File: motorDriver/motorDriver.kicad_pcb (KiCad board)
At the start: 2 copper layers, 20.1 x 21.3 mm, 8 parts, among them P1 Vcc, P2 Input, P3 Output, U1 TB6593FNG

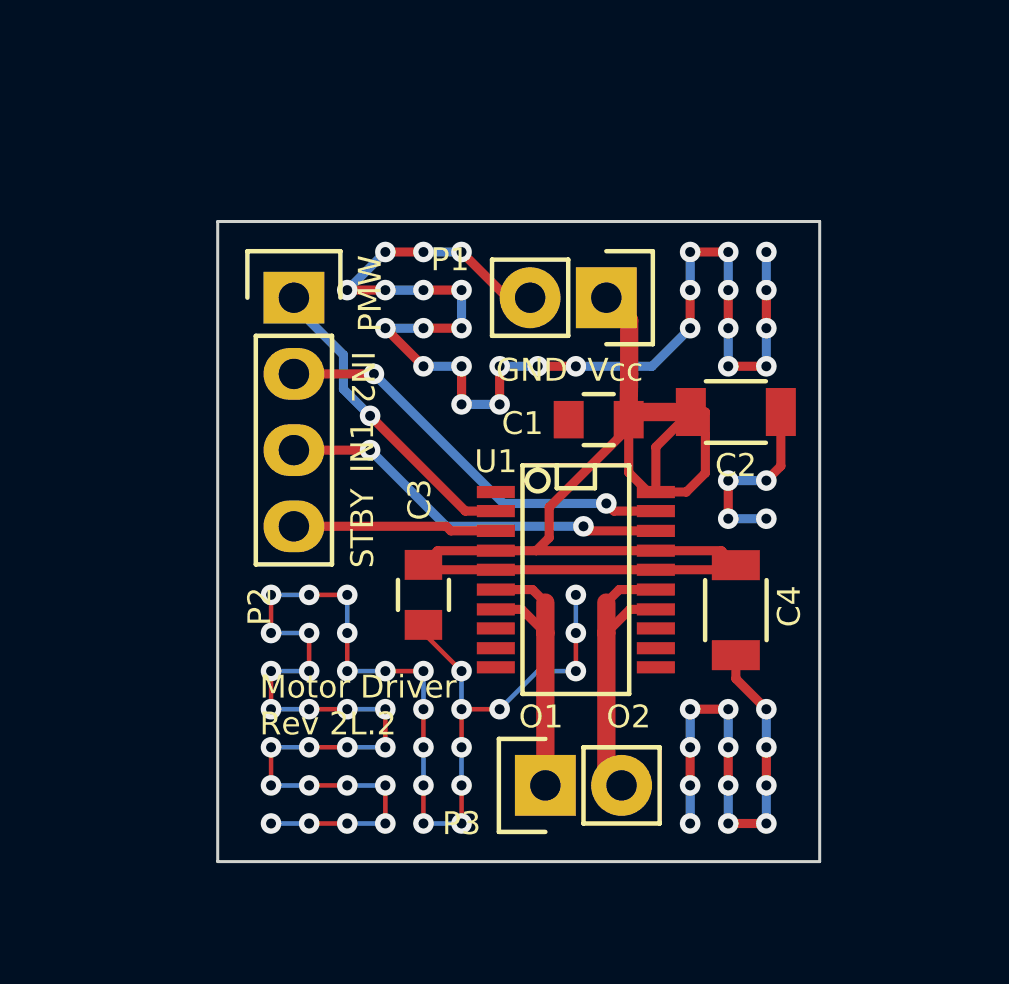
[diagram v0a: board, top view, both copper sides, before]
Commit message: Updated layout for Rev 2
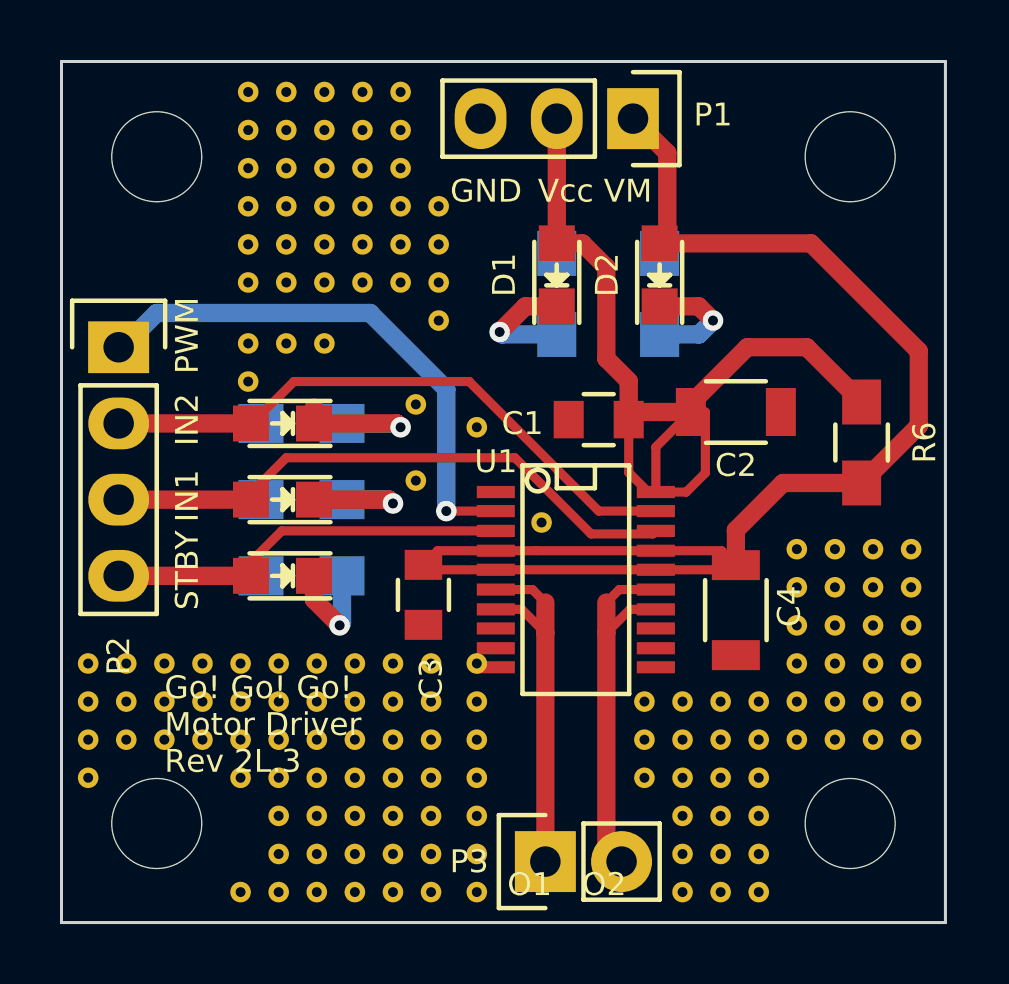
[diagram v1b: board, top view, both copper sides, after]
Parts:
- added D1: LED, LEDs:LED-0805, F.Cu at (159.4, 82.0)
- added D2: LED, LEDs:LED-0805, F.Cu at (162.8, 82.0)
- added D3: LED, LEDs:LED-0805, F.Cu at (150.2, 92.1)
- added IN1: LED, LEDs:LED-0805, F.Cu at (150.2, 89.5)
- added IN2: LED, LEDs:LED-0805, F.Cu at (150.2, 87.0)
- added R1: 1KΩ, Resistors_SMD:R_0805_HandSoldering, B.Cu at (159.4, 82.7)
- added R2: 1KΩ, Resistors_SMD:R_0805_HandSoldering, B.Cu at (162.8, 82.7)
- added R3: 1KΩ, Resistors_SMD:R_0805_HandSoldering, B.Cu at (150.9, 89.5)
- added R4: 1KΩ, Resistors_SMD:R_0805_HandSoldering, B.Cu at (150.9, 87.0)
- added R5: 1KΩ, Resistors_SMD:R_0805_HandSoldering, B.Cu at (150.9, 92.1)
- added R6: 0Ω, Resistors_SMD:R_0805_HandSoldering, F.Cu at (169.5, 87.6)
- added REF**: MountingHole_3mm, Mounting_Holes:MountingHole_3mm, F.Cu at (169.2, 100.3)
- added REF**: MountingHole_3mm, Mounting_Holes:MountingHole_3mm, F.Cu at (146.1, 100.3)
- added REF**: MountingHole_3mm, Mounting_Holes:MountingHole_3mm, F.Cu at (146.1, 78.1)
- added REF**: MountingHole_3mm, Mounting_Holes:MountingHole_3mm, F.Cu at (169.2, 78.1)
- added REF**111: Via, GoGoGo:Via, F.Cu at (149.1, 75.9)
- added REF**111111: Via, GoGoGo:Via, F.Cu at (167.4, 91.2)
- added REF**1111111: Via, GoGoGo:Via, F.Cu at (162.3, 96.3)
- added REF**111111101: Via, GoGoGo:Via, F.Cu at (155.2, 95.0)
- added REF**11111111: Via, GoGoGo:Via, F.Cu at (143.8, 95.0)
- added REF**1111111101: Via, GoGoGo:Via, F.Cu at (155.2, 96.3)
- added REF**1111111102: Via, GoGoGo:Via, F.Cu at (155.2, 97.5)
- added REF**1111111103: Via, GoGoGo:Via, F.Cu at (155.2, 98.8)
- added REF**1111111104: Via, GoGoGo:Via, F.Cu at (155.2, 100.1)
- added REF**1111111105: Via, GoGoGo:Via, F.Cu at (155.2, 101.3)
- added REF**1111111106: Via, GoGoGo:Via, F.Cu at (155.2, 102.6)
- added REF**111111111: Via, GoGoGo:Via, F.Cu at (143.8, 96.3)
- added REF**111111112: Via, GoGoGo:Via, F.Cu at (143.8, 97.5)
- added REF**111111113: Via, GoGoGo:Via, F.Cu at (143.8, 98.8)
- added REF**111111121: Via, GoGoGo:Via, F.Cu at (145.0, 96.3)
- added REF**111111122: Via, GoGoGo:Via, F.Cu at (145.0, 97.5)
- added REF**111111126: Via, GoGoGo:Via, F.Cu at (156.7, 96.3)
- added REF**111111131: Via, GoGoGo:Via, F.Cu at (146.3, 96.3)
- added REF**111111132: Via, GoGoGo:Via, F.Cu at (146.3, 97.5)
- added REF**111111136: Via, GoGoGo:Via, F.Cu at (156.7, 97.5)
- added REF**111111137: Via, GoGoGo:Via, F.Cu at (156.7, 95.0)
- added REF**111111138: Via, GoGoGo:Via, F.Cu at (156.7, 102.6)
- added REF**111111141: Via, GoGoGo:Via, F.Cu at (147.6, 96.3)
- added REF**111111142: Via, GoGoGo:Via, F.Cu at (147.6, 97.5)
- added REF**111111146: Via, GoGoGo:Via, F.Cu at (156.7, 98.8)
- added REF**111111147: Via, GoGoGo:Via, F.Cu at (156.7, 100.1)
- added REF**111111148: Via, GoGoGo:Via, F.Cu at (156.7, 101.3)
- added REF**111111151: Via, GoGoGo:Via, F.Cu at (148.8, 96.3)
- added REF**111111152: Via, GoGoGo:Via, F.Cu at (148.8, 97.5)
- added REF**111111153: Via, GoGoGo:Via, F.Cu at (148.8, 98.8)
- added REF**111111156: Via, GoGoGo:Via, F.Cu at (148.8, 102.6)
- added REF**111111161: Via, GoGoGo:Via, F.Cu at (150.1, 96.3)
- added REF**111111162: Via, GoGoGo:Via, F.Cu at (150.1, 97.5)
- added REF**111111163: Via, GoGoGo:Via, F.Cu at (150.1, 98.8)
- added REF**111111164: Via, GoGoGo:Via, F.Cu at (150.1, 100.1)
- added REF**111111165: Via, GoGoGo:Via, F.Cu at (150.1, 101.3)
- added REF**111111166: Via, GoGoGo:Via, F.Cu at (150.1, 102.6)
- added REF**111111171: Via, GoGoGo:Via, F.Cu at (151.4, 96.3)
- added REF**111111172: Via, GoGoGo:Via, F.Cu at (151.4, 97.5)
- added REF**111111173: Via, GoGoGo:Via, F.Cu at (151.4, 98.8)
- added REF**111111174: Via, GoGoGo:Via, F.Cu at (151.4, 100.1)
- added REF**111111175: Via, GoGoGo:Via, F.Cu at (151.4, 101.3)
- added REF**111111176: Via, GoGoGo:Via, F.Cu at (151.4, 102.6)
- added REF**111111181: Via, GoGoGo:Via, F.Cu at (152.7, 96.3)
- added REF**111111182: Via, GoGoGo:Via, F.Cu at (152.7, 97.5)
- added REF**111111183: Via, GoGoGo:Via, F.Cu at (152.7, 98.8)
- added REF**111111184: Via, GoGoGo:Via, F.Cu at (152.7, 100.1)
- added REF**111111185: Via, GoGoGo:Via, F.Cu at (152.7, 101.3)
- added REF**111111186: Via, GoGoGo:Via, F.Cu at (152.7, 102.6)
- added REF**111111191: Via, GoGoGo:Via, F.Cu at (153.9, 96.3)
- added REF**111111192: Via, GoGoGo:Via, F.Cu at (153.9, 97.5)
- added REF**111111193: Via, GoGoGo:Via, F.Cu at (153.9, 98.8)
- added REF**111111194: Via, GoGoGo:Via, F.Cu at (153.9, 100.1)
- added REF**111111195: Via, GoGoGo:Via, F.Cu at (153.9, 101.3)
- added REF**111111196: Via, GoGoGo:Via, F.Cu at (153.9, 102.6)
- added REF**1111112: Via, GoGoGo:Via, F.Cu at (162.3, 97.5)
- added REF**11111121: Via, GoGoGo:Via, F.Cu at (145.0, 95.0)
- added REF**1111113: Via, GoGoGo:Via, F.Cu at (162.3, 98.8)
- added REF**11111131: Via, GoGoGo:Via, F.Cu at (146.3, 95.0)
- added REF**11111141: Via, GoGoGo:Via, F.Cu at (147.6, 95.0)
- added REF**11111151: Via, GoGoGo:Via, F.Cu at (148.8, 95.0)
- added REF**11111161: Via, GoGoGo:Via, F.Cu at (150.1, 95.0)
- added REF**11111171: Via, GoGoGo:Via, F.Cu at (151.4, 95.0)
- added REF**11111181: Via, GoGoGo:Via, F.Cu at (152.7, 95.0)
- added REF**11111191: Via, GoGoGo:Via, F.Cu at (153.9, 95.0)
- added REF**111112: Via, GoGoGo:Via, F.Cu at (167.4, 92.5)
- added REF**1111121: Via, GoGoGo:Via, F.Cu at (163.6, 96.3)
- added REF**1111122: Via, GoGoGo:Via, F.Cu at (163.6, 97.5)
- added REF**1111123: Via, GoGoGo:Via, F.Cu at (163.6, 98.8)
- added REF**1111124: Via, GoGoGo:Via, F.Cu at (163.6, 100.1)
- added REF**1111125: Via, GoGoGo:Via, F.Cu at (163.6, 101.3)
- added REF**1111126: Via, GoGoGo:Via, F.Cu at (163.6, 102.6)
- added REF**111113: Via, GoGoGo:Via, F.Cu at (167.4, 93.7)
- added REF**1111131: Via, GoGoGo:Via, F.Cu at (164.8, 96.3)
- added REF**1111132: Via, GoGoGo:Via, F.Cu at (164.8, 97.5)
- added REF**1111133: Via, GoGoGo:Via, F.Cu at (164.8, 98.8)
- added REF**1111134: Via, GoGoGo:Via, F.Cu at (164.8, 100.1)
- added REF**1111135: Via, GoGoGo:Via, F.Cu at (164.8, 101.3)
- added REF**1111136: Via, GoGoGo:Via, F.Cu at (164.8, 102.6)
- added REF**111114: Via, GoGoGo:Via, F.Cu at (167.4, 95.0)
- added REF**1111141: Via, GoGoGo:Via, F.Cu at (166.1, 96.3)
- added REF**1111142: Via, GoGoGo:Via, F.Cu at (166.1, 97.5)
- added REF**1111143: Via, GoGoGo:Via, F.Cu at (166.1, 98.8)
- added REF**1111144: Via, GoGoGo:Via, F.Cu at (166.1, 100.1)
- added REF**1111145: Via, GoGoGo:Via, F.Cu at (166.1, 101.3)
- added REF**1111146: Via, GoGoGo:Via, F.Cu at (166.1, 102.6)
- added REF**111115: Via, GoGoGo:Via, F.Cu at (167.4, 96.3)
- added REF**111116: Via, GoGoGo:Via, F.Cu at (167.4, 97.5)
- added REF**111121: Via, GoGoGo:Via, F.Cu at (168.7, 91.2)
- added REF**111122: Via, GoGoGo:Via, F.Cu at (168.7, 92.5)
- added REF**111123: Via, GoGoGo:Via, F.Cu at (168.7, 93.7)
- added REF**111124: Via, GoGoGo:Via, F.Cu at (168.7, 95.0)
- added REF**111125: Via, GoGoGo:Via, F.Cu at (168.7, 96.3)
- added REF**111126: Via, GoGoGo:Via, F.Cu at (168.7, 97.5)
- added REF**111131: Via, GoGoGo:Via, F.Cu at (169.9, 91.2)
- added REF**111132: Via, GoGoGo:Via, F.Cu at (169.9, 92.5)
- added REF**111133: Via, GoGoGo:Via, F.Cu at (169.9, 93.7)
- added REF**111134: Via, GoGoGo:Via, F.Cu at (169.9, 95.0)
- added REF**111135: Via, GoGoGo:Via, F.Cu at (169.9, 96.3)
- added REF**111136: Via, GoGoGo:Via, F.Cu at (169.9, 97.5)
- added REF**111141: Via, GoGoGo:Via, F.Cu at (171.2, 91.2)
- added REF**111142: Via, GoGoGo:Via, F.Cu at (171.2, 92.5)
- added REF**111143: Via, GoGoGo:Via, F.Cu at (171.2, 93.7)
- added REF**111144: Via, GoGoGo:Via, F.Cu at (171.2, 95.0)
- added REF**111145: Via, GoGoGo:Via, F.Cu at (171.2, 96.3)
- added REF**111146: Via, GoGoGo:Via, F.Cu at (171.2, 97.5)
- added REF**112: Via, GoGoGo:Via, F.Cu at (149.1, 77.2)
- added REF**113: Via, GoGoGo:Via, F.Cu at (149.1, 78.5)
- added REF**114: Via, GoGoGo:Via, F.Cu at (149.1, 79.8)
- added REF**115: Via, GoGoGo:Via, F.Cu at (149.1, 81.0)
- added REF**116: Via, GoGoGo:Via, F.Cu at (149.1, 82.3)
- added REF**118: Via, GoGoGo:Via, F.Cu at (156.7, 87.1)
- added REF**118: Via, GoGoGo:Via, F.Cu at (154.7, 86.4)
- added REF**118: Via, GoGoGo:Via, F.Cu at (158.9, 90.3)
- added REF**118: Via, GoGoGo:Via, F.Cu at (151.6, 84.3)
- added REF**118: Via, GoGoGo:Via, F.Cu at (149.1, 85.6)
- added REF**118: Via, GoGoGo:Via, F.Cu at (150.4, 84.3)
- added REF**118: Via, GoGoGo:Via, F.Cu at (154.7, 88.9)
- added REF**118: Via, GoGoGo:Via, F.Cu at (149.1, 84.3)
- added REF**121: Via, GoGoGo:Via, F.Cu at (150.4, 75.9)
- added REF**122: Via, GoGoGo:Via, F.Cu at (150.4, 77.2)
- added REF**123: Via, GoGoGo:Via, F.Cu at (150.4, 78.5)
- added REF**124: Via, GoGoGo:Via, F.Cu at (150.4, 79.8)
- added REF**125: Via, GoGoGo:Via, F.Cu at (150.4, 81.0)
- added REF**126: Via, GoGoGo:Via, F.Cu at (150.4, 82.3)
- added REF**128: Via, GoGoGo:Via, F.Cu at (155.4, 83.6)
- added REF**131: Via, GoGoGo:Via, F.Cu at (151.6, 75.9)
- added REF**132: Via, GoGoGo:Via, F.Cu at (151.6, 77.2)
- added REF**133: Via, GoGoGo:Via, F.Cu at (151.6, 78.5)
- added REF**134: Via, GoGoGo:Via, F.Cu at (151.6, 79.8)
- added REF**135: Via, GoGoGo:Via, F.Cu at (151.6, 81.0)
- added REF**136: Via, GoGoGo:Via, F.Cu at (151.6, 82.3)
- added REF**138: Via, GoGoGo:Via, F.Cu at (155.4, 82.3)
- added REF**141: Via, GoGoGo:Via, F.Cu at (152.9, 75.9)
- added REF**142: Via, GoGoGo:Via, F.Cu at (152.9, 77.2)
- added REF**143: Via, GoGoGo:Via, F.Cu at (152.9, 78.5)
- added REF**144: Via, GoGoGo:Via, F.Cu at (152.9, 79.8)
- added REF**145: Via, GoGoGo:Via, F.Cu at (152.9, 81.0)
- added REF**146: Via, GoGoGo:Via, F.Cu at (152.9, 82.3)
- added REF**148: Via, GoGoGo:Via, F.Cu at (155.4, 81.0)
- added REF**151: Via, GoGoGo:Via, F.Cu at (154.2, 75.9)
- added REF**152: Via, GoGoGo:Via, F.Cu at (154.2, 77.2)
- added REF**153: Via, GoGoGo:Via, F.Cu at (154.2, 78.5)
- added REF**154: Via, GoGoGo:Via, F.Cu at (154.2, 79.8)
- added REF**155: Via, GoGoGo:Via, F.Cu at (154.2, 81.0)
- added REF**156: Via, GoGoGo:Via, F.Cu at (154.2, 82.3)
- added REF**158: Via, GoGoGo:Via, F.Cu at (155.4, 79.8)
- P1: value Vcc -> CONN_01X03; footprint Pin_Headers:Pin_Header_Straight_1x02 -> Pin_Headers:Pin_Header_Straight_1x03
- moved P2 6.07 mm to (144.8, 84.5)
- moved P1 6.03 mm to (161.9, 76.8)
- moved P3 2.54 mm to (159.0, 101.6)
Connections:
- C1 pad 1: /VM -> /Vcc
- C2 pad 1: /VM -> /Vcc
- P1 pad 2: GND -> /Vcc
- U1 pad 20: /VM -> /Vcc
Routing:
- net GND: track 117.2 -> 0.27 mm, vias 84 -> 0
- net /Vcc: track 0.00 -> 32.9 mm
- net /PMW: track 11.3 -> 19.2 mm
- net /IN1: track 13.2 -> 19.2 mm, vias 2 -> 0
- net /STBY: track 7.15 -> 12.8 mm
- net /IN2: track 14.0 -> 19.5 mm, vias 2 -> 0
- net Net-(IN2-Pad1): track 0.00 -> 5.49 mm, vias 0 -> 1
- net Net-(IN1-Pad1): track 0.00 -> 4.44 mm, vias 0 -> 1
- net Net-(D1-Pad1): track 0.00 -> 4.20 mm, vias 0 -> 1
- net Net-(D2-Pad1): track 0.00 -> 3.94 mm, vias 0 -> 1
- net Net-(D3-Pad1): track 0.00 -> 3.69 mm, vias 0 -> 1
- net /VM: track 44.6 -> 47.7 mm
- net /O2: track 10.1 -> 12.7 mm
- net /O1: track 9.90 -> 12.4 mm
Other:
- board size 20.1 x 21.3 mm -> 29.5 x 28.7 mm
- board text added: "Go! Go! Go! Motor Driver Rev 2L.3"
- board text added: "O1 O2"
- board text added: "PWM"
- board text added: "Vcc VM"
- board text removed: "IN1"
- board text removed: "IN2"
- board text removed: "Motor Driver Rev 2L.2"
- board text removed: "O1"
- board text removed: "O2"
- board text removed: "PMW"
- board text removed: "Vcc"
